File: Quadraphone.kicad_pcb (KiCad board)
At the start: 4 copper layers, 60 x 100 mm, 185 parts, among them J1 Conn_01x10_Male, J2 Conn_01x10_Male, J3 Conn_01x10_Male, J4 Conn_01x10_Male, J5 Eurorack_10_pin_power, U1 AMS1117-5.0, U10 TL072, U11 4066, U12 SSI2131, U13 TL072, U14 LM4040DBZ-2.5, U15 4066, U16 TL072, U17 SSI2131, U18 TL072, U22 SSI2131, U3 MCP6002, U4 LM4040DBZ-5, U5 MCP6004, U6 4066, U7 4066, U8 4066, U9 SSI2131

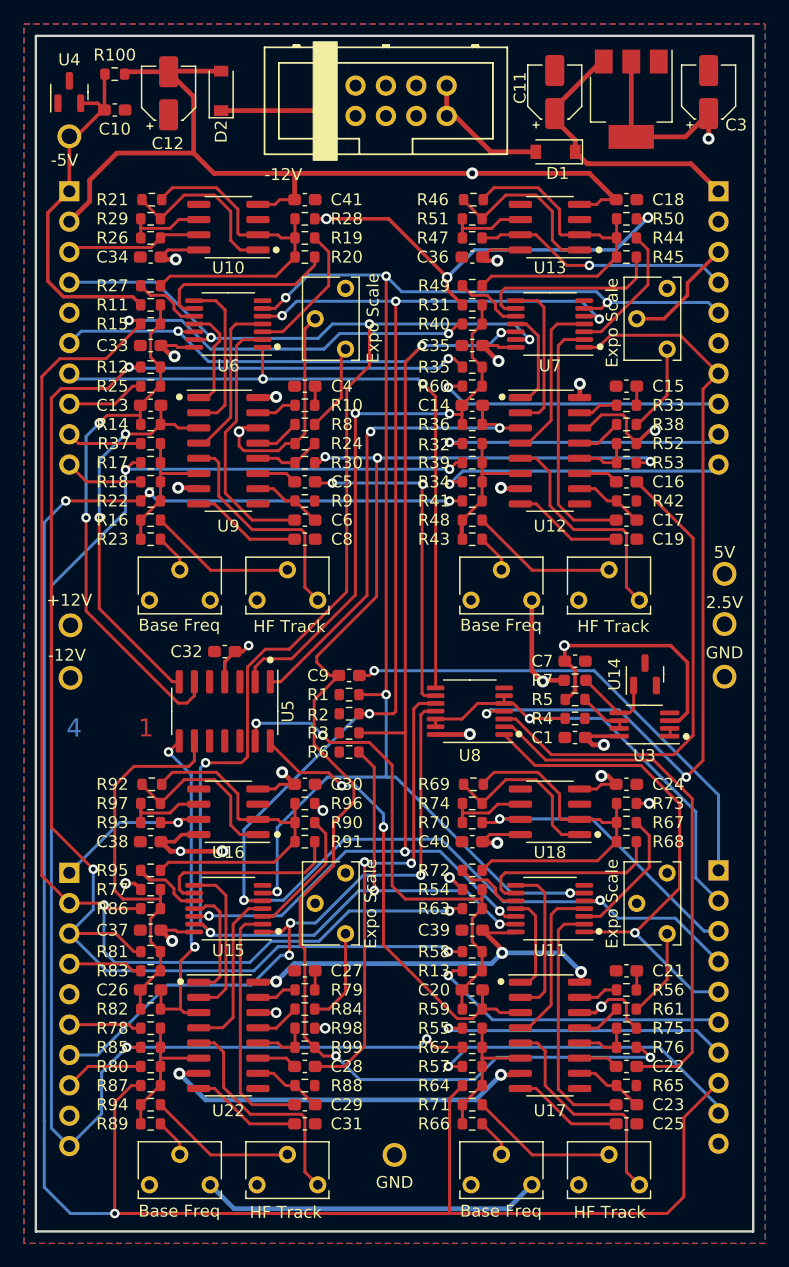
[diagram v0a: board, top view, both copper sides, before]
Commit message: First draft panel done
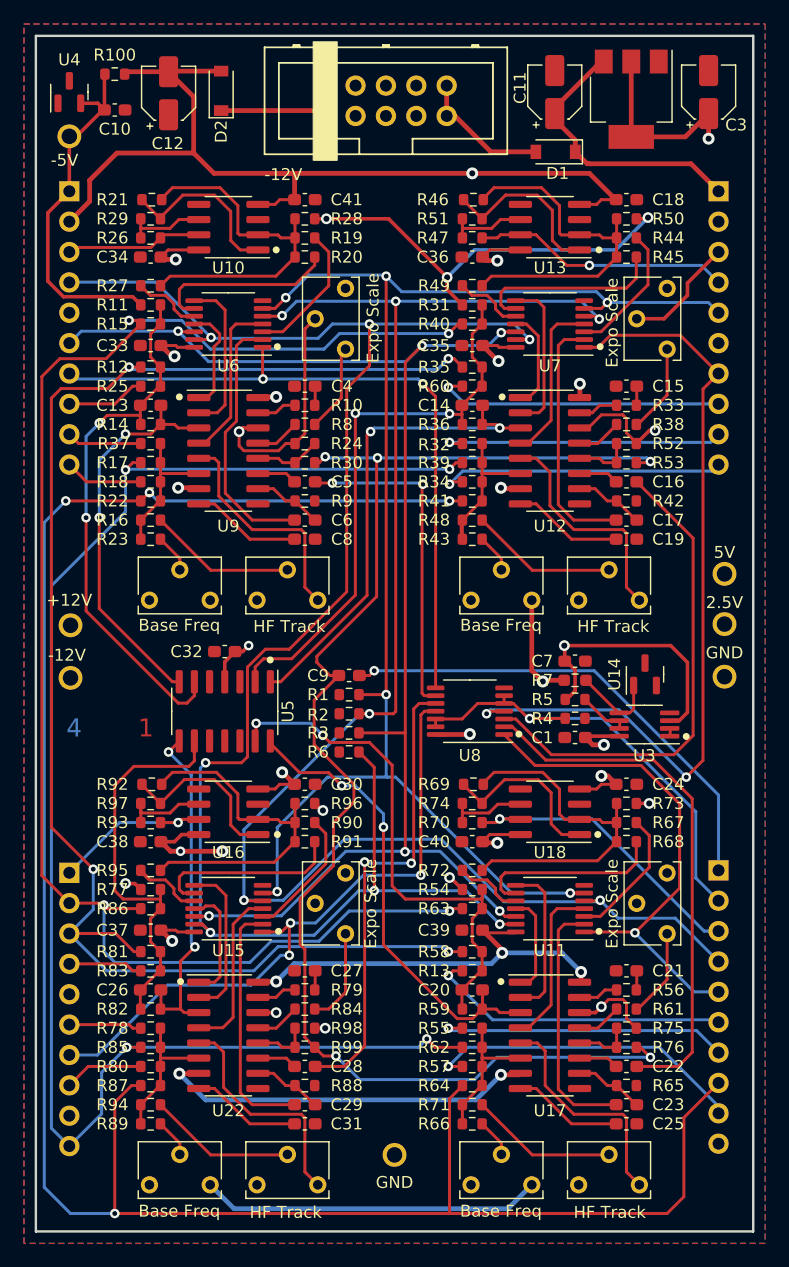
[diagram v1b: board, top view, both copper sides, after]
